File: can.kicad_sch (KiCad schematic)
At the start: 18 parts, among them U1 SN6501DBVR, U2 ISO1050DWR, U3 TPS76350DBVR

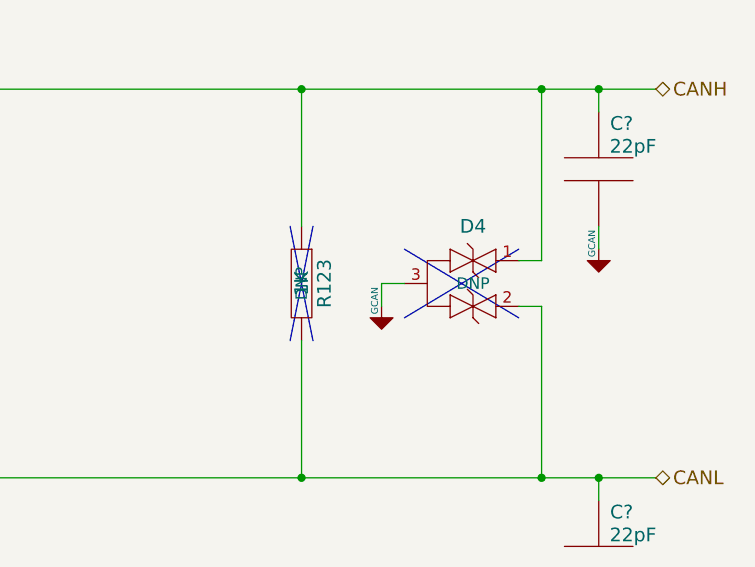
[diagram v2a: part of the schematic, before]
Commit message: assy
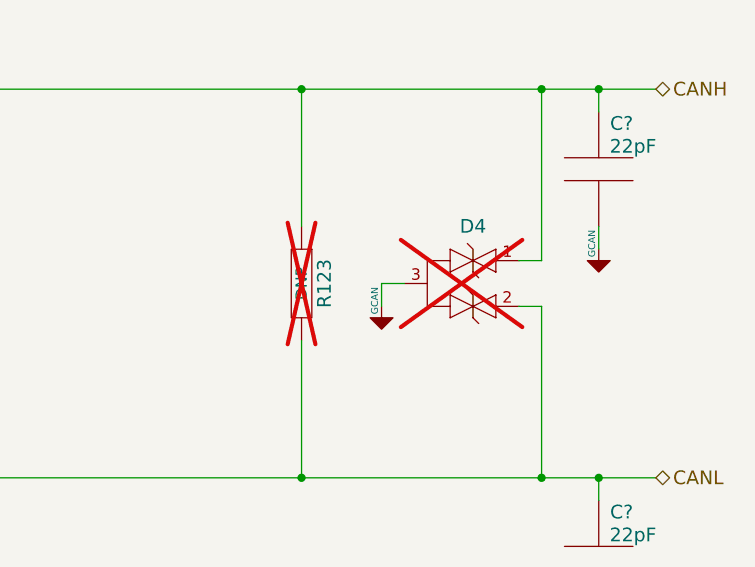
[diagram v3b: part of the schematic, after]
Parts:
- D4, R123: now not fitted
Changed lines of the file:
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@@
-    (stroke (width 0) (type default))
-  )
-  (polyline (pts (xy 242.57 148.59) (xy 255.27 140.97))
     (stroke (width 0) (type default))
   )
@@
     (stroke (width 0) (type default))
   )
-  (polyline (pts (xy 242.57 140.97) (xy 255.27 148.59))
-    (stroke (width 0) (type default))
-  )
   (wire (pts (xy 115.57 78.74) (xy 110.49 78.74))
     (stroke (width 0) (type default))
@@
     (stroke (width 0) (type default))
   )
-  (polyline (pts (xy 229.87 151.13) (xy 232.41 138.43))
-    (stroke (width 0) (type default))
-  )
   (wire (pts (xy 59.69 59.69) (xy 59.69 71.12))
     (stroke (width 0) (type default))
@@
   )
   (wire (pts (xy 264.16 166.37) (xy 257.81 166.37))
-    (stroke (width 0) (type default))
-  )
-  (polyline (pts (xy 229.87 138.43) (xy 232.41 151.13))
     (stroke (width 0) (type default))
   )
@@
   )
   (symbol (lib_id "Resistor_Yageo:RC0603FR-071KL") (at 231.14 144.78 270) (unit 1)
-    (in_bom yes) (on_board yes) (dnp no)
+    (in_bom yes) (on_board yes) (dnp yes)
     (property "Reference" "R123" (at 233.68 144.78 0)
       (effects (font (size 1.524 1.524)))
@@
     )
     (property "Nominal" "1K" (at 231.14 144.78 0)
-      (effects (font (size 1.524 1.524)))
+      (effects (font (size 1.524 1.524)) hide)
     )
     (property "Tolerance" "1%" (at 213.995 144.78 0)
@@
     (property "SupplierPartNumber" "311-1.00KHRTR-ND" (at 223.52 144.78 0)
       (effects (font (size 1.524 1.524)) hide)
+    )
+    (property "Variant" "" (at 231.14 144.78 0)
+      (effects (font (size 1.27 1.27)) hide)
     )
     (pin "1")
@@
   )
   (symbol (lib_id "STMicroelectronics:ESDCAN05-2BWY") (at 250.19 144.78 0) (mirror y) (unit 1)
-    (in_bom yes) (on_board yes) (dnp no)
+    (in_bom yes) (on_board yes) (dnp yes)
     (property "Reference" "D4" (at 250.19 138.43 0)
       (effects (font (size 1.524 1.524)))
@@
     )
     (property "fit_field" "DNP" (at 250.19 144.78 0)
-      (effects (font (size 1.27 1.27)))
-    )
-    (pin "1")
+      (effects (font (size 1.27 1.27)) hide)
+    )
+    (property "Variant" "" (at 250.19 144.78 0)
+      (effects (font (size 1.27 1.27)) hide)
+    )
+    (property "Nominal" "" (at 250.19 144.78 0)
+      (effects (font (size 1.27 1.27)) hide)
+    )
+    (property "Power" "" (at 250.19 144.78 0)
+      (effects (font (size 1.27 1.27)) hide)
+    )
+    (pin "1")

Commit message: - zero origin on so - silk - sch trig and rtsi lines need 510 resistor - assembly updated - sch and pcb project name and rev - no changes to gerber, old one can be used
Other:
- title: EOL ECU POWER CARD -> EOL ECU MIX CARD
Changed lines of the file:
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@@
   (paper "A3")
   (title_block
-    (title "EOL ECU POWER CARD")
-    (date "2023-04-03")
-    (rev "0B")
+    (title "EOL ECU MIX CARD")
+    (date "2023-09-26")
+    (rev "0C")
     (company "ARXTRON TECHNOLOGIES")
     (comment 1 "A0180-V0")

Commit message: pnp added
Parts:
- D4, R123: now left out of the parts list
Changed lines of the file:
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@@
-(kicad_sch (version 20230620) (generator eeschema)
+(kicad_sch (version 20230819) (generator eeschema)
   (paper "A3")
   (title_block
@@
   )
   (symbol (lib_id "Resistor_Yageo:RC0603FR-071KL") (at 231.14 144.78 270) (unit 1)
-    (in_bom yes) (on_board yes) (dnp yes)
+    (exclude_from_sim no) (in_bom no) (on_board yes) (dnp yes)
     (property "Reference" "R123" (at 233.68 144.78 0)
       (effects (font (size 1.524 1.524)))
@@
   )
   (symbol (lib_id "_power_symbol:GND_CAN") (at 264.16 140.97 0) (unit 1)
-    (in_bom yes) (on_board yes) (dnp no)
+    (exclude_from_sim no) (in_bom yes) (on_board yes) (dnp no)
     (property "Reference" "#PWR?" (at 264.16 147.32 0)
       (effects (font (size 1.27 1.27)) hide)
@@
   )
   (symbol (lib_id "_power_symbol:GND_CAN") (at 264.16 184.15 0) (unit 1)
-    (in_bom yes) (on_board yes) (dnp no)
+    (exclude_from_sim no) (in_bom yes) (on_board yes) (dnp no)
     (property "Reference" "#PWR?" (at 264.16 190.5 0)
       (effects (font (size 1.27 1.27)) hide)
@@
   )
   (symbol (lib_id "Capacitor_AVX:06035C104KAZ2A") (at 85.09 119.38 270) (unit 1)
-    (in_bom yes) (on_board yes) (dnp no)
+    (exclude_from_sim no) (in_bom yes) (on_board yes) (dnp no)
     (property "Reference" "C17" (at 86.36 114.3 90)
       (effects (font (size 1.524 1.524)) (justify left))
@@
   )
   (symbol (lib_id "Resistor_Yageo:RC0805FR-072KL") (at 50.8 129.54 270) (unit 1)
-    (in_bom yes) (on_board yes) (dnp no)
+    (exclude_from_sim no) (in_bom yes) (on_board yes) (dnp no)
     (property "Reference" "R114" (at 53.34 129.54 0)
       (effects (font (size 1.524 1.524)))
@@
   )
   (symbol (lib_id "Capacitor_AVX:12103C106KAT2A") (at 110.49 96.52 270) (unit 1)
-    (in_bom yes) (on_board yes) (dnp no)
+    (exclude_from_sim no) (in_bom yes) (on_board yes) (dnp no)
     (property "Reference" "C18" (at 113.03 92.71 90)
       (effects (font (size 1.524 1.524)))
@@
   )
   (symbol (lib_id "Capacitor_AVX:12103C106KAT2A") (at 229.87 82.55 270) (unit 1)
-    (in_bom yes) (on_board yes) (dnp no)
+    (exclude_from_sim no) (in_bom yes) (on_board yes) (dnp no)
     (property "Reference" "C21" (at 232.41 78.74 90)
       (effects (font (size 1.524 1.524)))
@@
   )
   (symbol (lib_id "Capacitor_AVX:12103C106KAT2A") (at 160.02 82.55 270) (unit 1)
-    (in_bom yes) (on_board yes) (dnp no)
+    (exclude_from_sim no) (in_bom yes) (on_board yes) (dnp no)
     (property "Reference" "C20" (at 162.56 78.74 90)
       (effects (font (size 1.524 1.524)))
@@
   )
   (symbol (lib_id "_power_symbol:GND_CAN") (at 160.02 91.44 0) (unit 1)
-    (in_bom yes) (on_board yes) (dnp no)
+    (exclude_from_sim no) (in_bom yes) (on_board yes) (dnp no)
     (property "Reference" "#PWR?" (at 160.02 97.79 0)
       (effects (font (size 1.27 1.27)) hide)
@@
   )
   (symbol (lib_id "_power_symbol:GND_CAN") (at 170.18 91.44 0) (unit 1)
-    (in_bom yes) (on_board yes) (dnp no)
+    (exclude_from_sim no) (in_bom yes) (on_board yes) (dnp no)
     (property "Reference" "#PWR?" (at 170.18 97.79 0)
       (effects (font (size 1.27 1.27)) hide)
@@
   )
   (symbol (lib_id "_power_symbol:GND_CAN") (at 180.34 91.44 0) (unit 1)
-    (in_bom yes) (on_board yes) (dnp no)
+    (exclude_from_sim no) (in_bom yes) (on_board yes) (dnp no)
     (property "Reference" "#PWR?" (at 180.34 97.79 0)
       (effects (font (size 1.27 1.27)) hide)
@@
   )
   (symbol (lib_id "_power_symbol:GND_CAN") (at 160.02 124.46 0) (unit 1)
-    (in_bom yes) (on_board yes) (dnp no)
+    (exclude_from_sim no) (in_bom yes) (on_board yes) (dnp no)
     (property "Reference" "#PWR?" (at 160.02 130.81 0)
       (effects (font (size 1.27 1.27)) hide)
@@
   )
   (symbol (lib_id "_power_symbol:GND_CAN") (at 229.87 91.44 0) (unit 1)
-    (in_bom yes) (on_board yes) (dnp no)
+    (exclude_from_sim no) (in_bom yes) (on_board yes) (dnp no)
     (property "Reference" "#PWR?" (at 229.87 97.79 0)
       (effects (font (size 1.27 1.27)) hide)
@@
   )
   (symbol (lib_id "_power_symbol:GND_CAN") (at 240.03 147.32 0) (unit 1)
-    (in_bom yes) (on_board yes) (dnp no)
+    (exclude_from_sim no) (in_bom yes) (on_board yes) (dnp no)
     (property "Reference" "#PWR?" (at 240.03 153.67 0)
       (effects (font (size 1.27 1.27)) hide)
@@
   )
   (symbol (lib_id "_power_symbol:GND_CAN") (at 143.51 156.21 0) (unit 1)
-    (in_bom yes) (on_board yes) (dnp no)
+    (exclude_from_sim no) (in_bom yes) (on_board yes) (dnp no)
     (property "Reference" "#PWR?" (at 143.51 162.56 0)
       (effects (font (size 1.27 1.27)) hide)
@@
   )
   (symbol (lib_id "_power_symbol:GND_CAN") (at 128.27 91.44 0) (unit 1)
-    (in_bom yes) (on_board yes) (dnp no)
+    (exclude_from_sim no) (in_bom yes) (on_board yes) (dnp no)
     (property "Reference" "#PWR?" (at 128.27 97.79 0)
       (effects (font (size 1.27 1.27)) hide)
@@
   )
   (symbol (lib_id "TI:SN6501DBVR") (at 88.9 88.9 0) (unit 1)
-    (in_bom yes) (on_board yes) (dnp no)
+    (exclude_from_sim no) (in_bom yes) (on_board yes) (dnp no)
     (property "Reference" "U1" (at 88.9 69.85 0)
       (effects (font (size 1.524 1.524)))
@@
   )
   (symbol (lib_id "TI:TPS76350DBVR") (at 200.66 82.55 0) (unit 1)
-    (in_bom yes) (on_board yes) (dnp no)
+    (exclude_from_sim no) (in_bom yes) (on_board yes) (dnp no)
     (property "Reference" "U3" (at 200.66 69.85 0)
       (effects (font (size 1.524 1.524)))
@@
   )
   (symbol (lib_id "TI:ISO1050DWR") (at 120.65 152.4 0) (unit 1)
-    (in_bom yes) (on_board yes) (dnp no)
+    (exclude_from_sim no) (in_bom yes) (on_board yes) (dnp no)
     (property "Reference" "U2" (at 123.19 128.27 0)
       (effects (font (size 1.524 1.524)))
@@
   )
   (symbol (lib_id "OnSemiconductor:SBR80520LT1G") (at 137.16 73.66 0) (unit 1)
-    (in_bom yes) (on_board yes) (dnp no)
+    (exclude_from_sim no) (in_bom yes) (on_board yes) (dnp no)
     (property "Reference" "D2" (at 137.16 71.12 0)
       (effects (font (size 1.524 1.524)))
@@
   )
   (symbol (lib_id "OnSemiconductor:SBR80520LT1G") (at 137.16 83.82 0) (unit 1)
-    (in_bom yes) (on_board yes) (dnp no)
+    (exclude_from_sim no) (in_bom yes) (on_board yes) (dnp no)
     (property "Reference" "D3" (at 137.16 81.28 0)
       (effects (font (size 1.524 1.524)))
@@
   )
   (symbol (lib_id "STMicroelectronics:ESDCAN05-2BWY") (at 250.19 144.78 0) (mirror y) (unit 1)
-    (in_bom yes) (on_board yes) (dnp yes)
+    (exclude_from_sim no) (in_bom no) (on_board yes) (dnp yes)
     (property "Reference" "D4" (at 250.19 138.43 0)
       (effects (font (size 1.524 1.524)))
@@
   )
   (symbol (lib_id "Capacitor_AVX:06035C104KAZ2A") (at 59.69 77.47 270) (unit 1)
-    (in_bom yes) (on_board yes) (dnp no)
+    (exclude_from_sim no) (in_bom yes) (on_board yes) (dnp no)
     (property "Reference" "C14" (at 60.96 72.39 90)
       (effects (font (size 1.524 1.524)) (justify left))
@@
   )
   (symbol (lib_id "Wurth:760390015") (at 120.65 78.74 0) (unit 1)
-    (in_bom yes) (on_board yes) (dnp no)
+    (exclude_from_sim no) (in_bom yes) (on_board yes) (dnp no)
     (property "Reference" "TR1" (at 120.65 63.5 0)
       (effects (font (size 1.524 1.524)))
@@
   )
   (symbol (lib_id "_power_symbol:GND_3V3") (at 68.58 86.36 0) (unit 1)
-    (in_bom yes) (on_board yes) (dnp no)
+    (exclude_from_sim no) (in_bom yes) (on_board yes) (dnp no)
     (property "Reference" "#PWR045" (at 68.58 92.71 0)
       (effects (font (size 1.27 1.27)) hide)
@@
   )
   (symbol (lib_id "_power_symbol:GND_3V3") (at 110.49 105.41 0) (unit 1)
-    (in_bom yes) (on_board yes) (dnp no)
+    (exclude_from_sim no) (in_bom yes) (on_board yes) (dnp no)
     (property "Reference" "#PWR047" (at 110.49 111.76 0)
       (effects (font (size 1.27 1.27)) hide)
@@
   )
   (symbol (lib_id "_power_symbol:GND_3V3") (at 59.69 86.36 0) (unit 1)
-    (in_bom yes) (on_board yes) (dnp no)
+    (exclude_from_sim no) (in_bom yes) (on_board yes) (dnp no)
     (property "Reference" "#PWR046" (at 59.69 92.71 0)
       (effects (font (size 1.27 1.27)) hide)
@@
   )
   (symbol (lib_id "Capacitor_AVX:06035C104KAZ2A") (at 170.18 82.55 270) (unit 1)
-    (in_bom yes) (on_board yes) (dnp no)
+    (exclude_from_sim no) (in_bom yes) (on_board yes) (dnp no)
     (property "Reference" "C22" (at 171.45 77.47 90)
       (effects (font (size 1.524 1.524)) (justify left))
@@
   )
   (symbol (lib_id "_power_symbol:GND_3V3") (at 100.33 156.21 0) (unit 1)
-    (in_bom yes) (on_board yes) (dnp no)
+    (exclude_from_sim no) (in_bom yes) (on_board yes) (dnp no)
     (property "Reference" "#PWR048" (at 100.33 162.56 0)
       (effects (font (size 1.27 1.27)) hide)
@@
   )
   (symbol (lib_id "_power_symbol:GND_3V3") (at 85.09 128.27 0) (unit 1)
-    (in_bom yes) (on_board yes) (dnp no)
+    (exclude_from_sim no) (in_bom yes) (on_board yes) (dnp no)
     (property "Reference" "#PWR049" (at 85.09 134.62 0)
       (effects (font (size 1.27 1.27)) hide)
@@
   )
   (symbol (lib_id "Capacitor_AVX:06035C104KAZ2A") (at 151.13 121.92 180) (unit 1)
-    (in_bom yes) (on_board yes) (dnp no)
+    (exclude_from_sim no) (in_bom yes) (on_board yes) (dnp no)
     (property "Reference" "C19" (at 156.21 123.19 90)
       (effects (font (size 1.524 1.524)) (justify left))
@@
   )
   (symbol (lib_id "Capacitor_AVX:08055A220JAT2A") (at 264.16 132.08 270) (unit 1)
-    (in_bom yes) (on_board yes) (dnp no)
+    (exclude_from_sim no) (in_bom yes) (on_board yes) (dnp no)
     (property "Reference" "C?" (at 266.7 127 90)
       (effects (font (size 1.524 1.524)))
@@
   )
   (symbol (lib_id "Capacitor_AVX:08055A220JAT2A") (at 264.16 175.26 270) (unit 1)
-    (in_bom yes) (on_board yes) (dnp no)
+    (exclude_from_sim no) (in_bom yes) (on_board yes) (dnp no)
     (property "Reference" "C?" (at 266.7 170.18 90)
       (effects (font (size 1.524 1.524)))
